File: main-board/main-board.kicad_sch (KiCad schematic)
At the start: 92 parts, among them IC13 TPS2121RUXR, J2 Conn_01x01_Socket, J47 Barrel Jack, J6 Conn_01x03, J66 Conn_01x01_Socket, J7 Conn_Boaxial, J73 Conn_01x03, J8 USB_C_Receptacle_USB2.0_16P, J9 Conn_02x04_Odd_Even, SW1 SW_Push, SW5 SW_Push, U10 SI5351A-B-GTR, U15 BIWIN_DTS04GE_SMD, U3 TLV75801PDBV, U4 MAX17577, U5 TLV75801PDBV, X1 OK322532.768KJBA4SL, Y2 NX3225GA-25.000M-STD-CRG-2

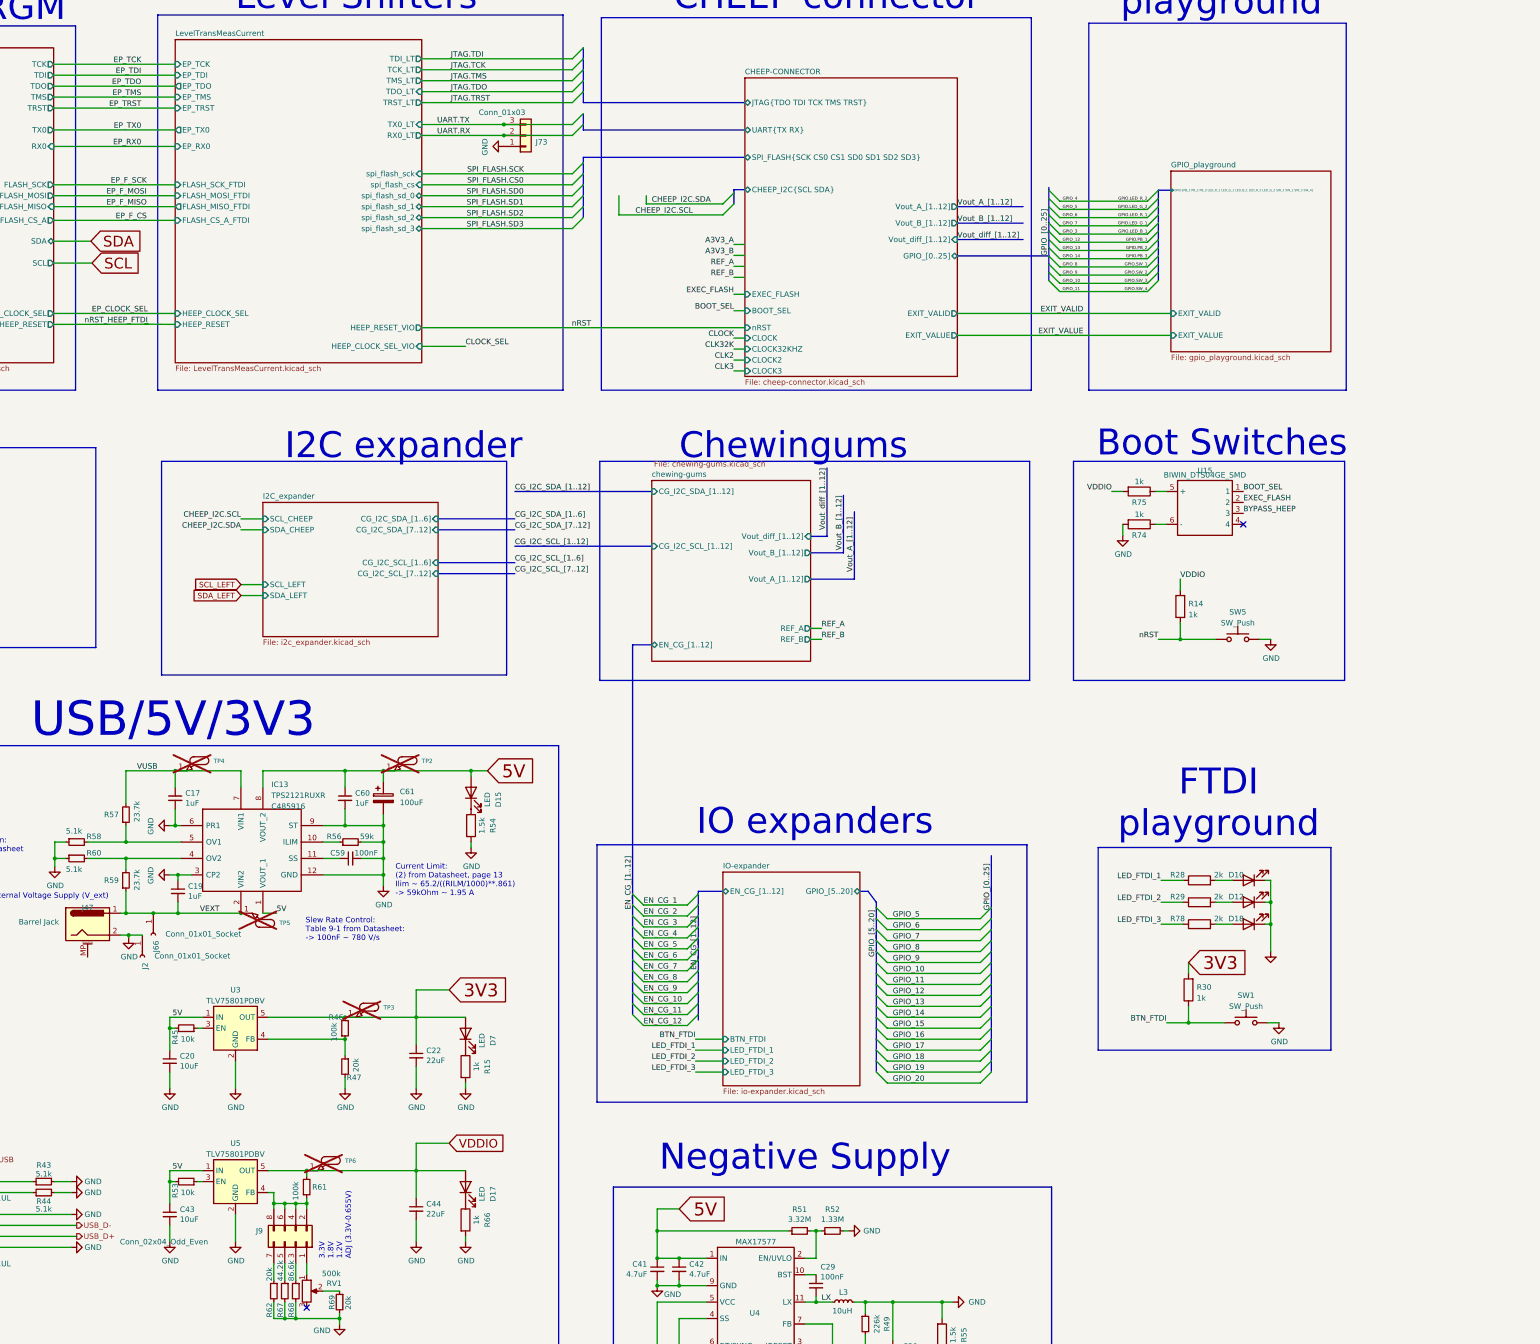
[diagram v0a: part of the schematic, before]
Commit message: Testing board final version & production data
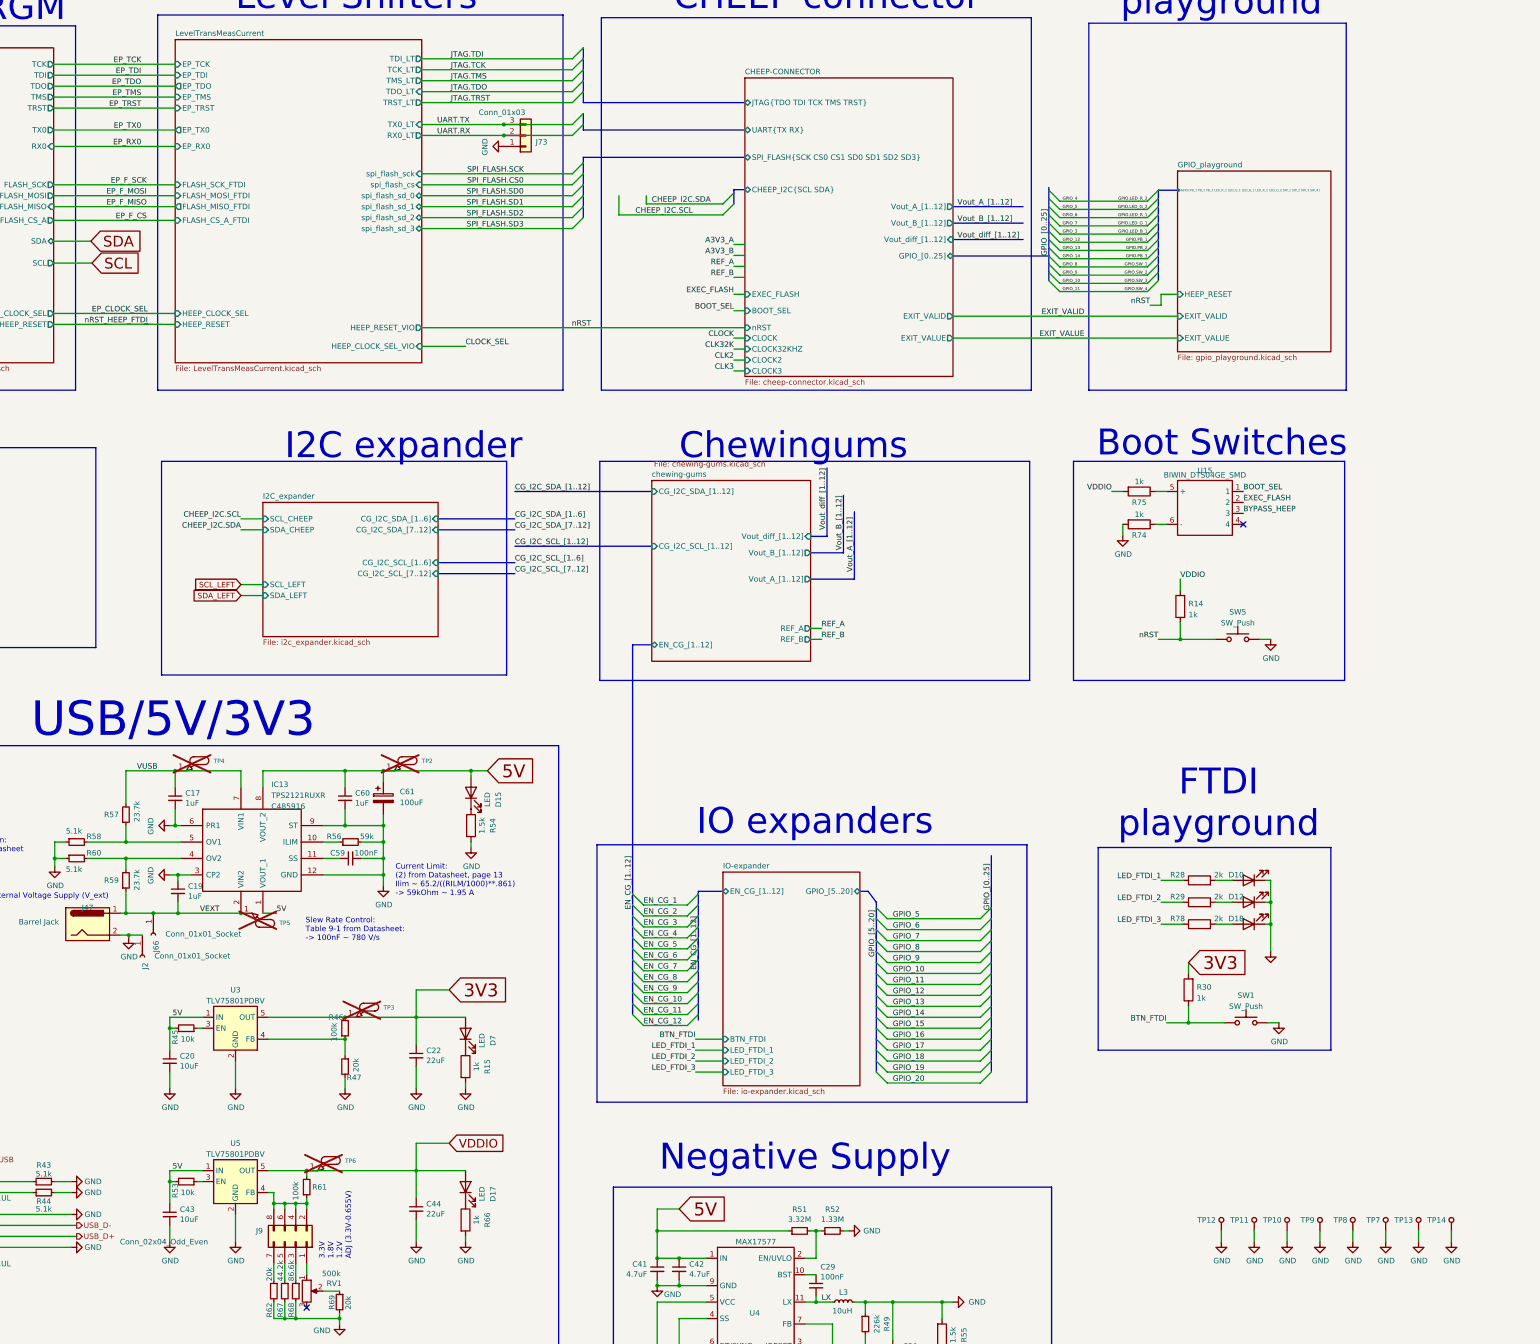
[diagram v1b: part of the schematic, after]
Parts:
- added TP10, TP11, TP12, TP13, TP14, TP7, TP8, TP9: 5029, TestPoint:TestPoint_Keystone_5019_Miniature, symbol dk_Test-Points:5029
- IC13: footprint SOTFL50P160X60-8N -> heep_footprints:TI-VQFN-HR-12
- J47: symbol Connector:Barrel_Jack_MountingPin -> Connector:Barrel_Jack
- L3: footprint Inductor_SMD:L_Coilcraft_XAL5030-XXX -> Inductor_SMD:L_Vishay_IHLP-2020
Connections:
- net GND: now also TP10.1, TP11.1, TP12.1, TP13.1, TP14.1, TP7.1, TP8.1, TP9.1
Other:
- sheet GPIO_playground ports: added HEEP_RESET; removed none

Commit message: production files
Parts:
- J6: LCSC C41417342 -> C5160786
- L3: LCSC C3911698 -> C844996
- U4: footprint Package_DFN_QFN:DFN-12-1EP_3x3mm_P0.45mm_EP1.65x2.38mm_ThermalVias -> heep_footprints:MAX17577-12-TDFN-EP
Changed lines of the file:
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@@
 			)
 		)
-		(property "LCSC" "C3911698"
+		(property "LCSC" "C844996"
 			(at 421.64 359.664 0)
 			(effects
@@
 			)
 		)
-		(property "LCSC" "C41417342"
+		(property "LCSC" "C5160786"
 			(at 65.786 302.641 0)
 			(effects
@@
 			)
 		)
-		(property "Footprint" "Package_DFN_QFN:DFN-12-1EP_3x3mm_P0.45mm_EP1.65x2.38mm_ThermalVias"
+		(property "Footprint" "heep_footprints:MAX17577-12-TDFN-EP"
 			(at 401.32 364.49 0)
 			(effects
